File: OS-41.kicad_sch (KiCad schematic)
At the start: 65 parts, among them J1 Conn_02x03_Counter_Clockwise, J2 Conn_01x02_Pin, J3 Conn_01x02_Pin, J4 Conn_Coaxial, SW4 SW_Push, U1 BME280, U2 SI4432-B1-FMR, U3 MCP1640x-xCHY, U4 ATGM336H-5N31, U7 STM32F103C8Tx, Y1 32.768KHz 12.5pF, Y2 8MHz 12pF, Y3 30MHz 10pF

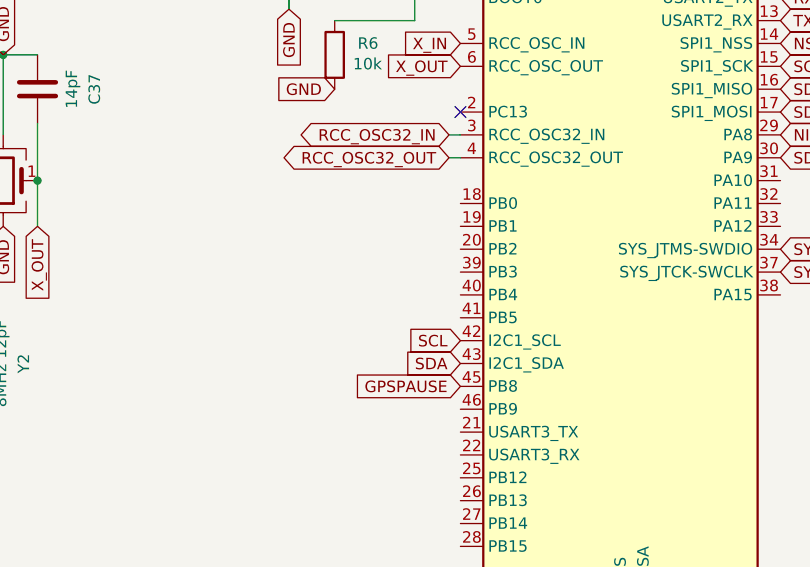
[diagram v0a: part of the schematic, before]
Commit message: Routed first version!
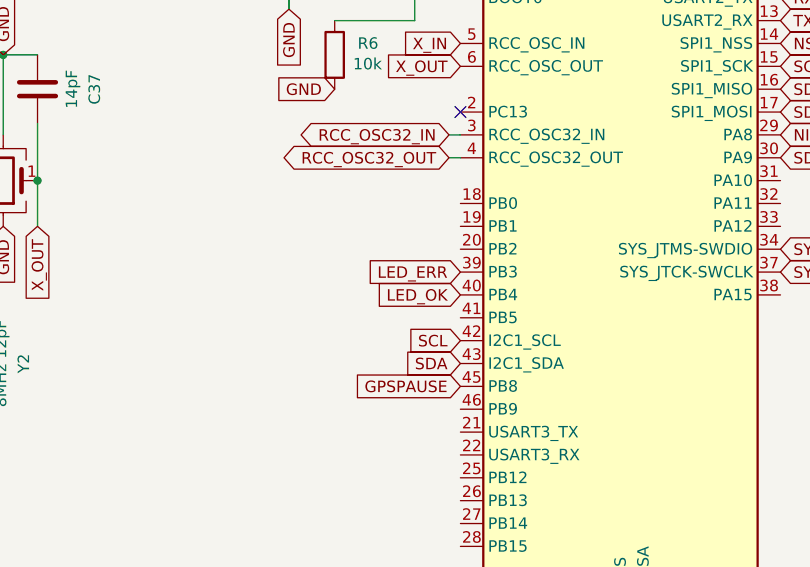
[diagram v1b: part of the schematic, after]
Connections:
- net LED_ERR: now also U7.39 (PB3)
- net LED_OK: now also U7.40 (PB4)
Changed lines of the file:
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@@
+		)
+	)
+	(global_label "LED_ERR"
+		(shape input)
+		(at 290.83 91.44 180)
+		(fields_autoplaced yes)
+		(effects
+			(font
+				(size 1.27 1.27)
+			)
+			(justify right)
+		)
+		(property "Intersheetrefs" "${INTERSHEET_REFS}"
+			(at 279.7411 91.44 0)
+			(effects
+				(font
+					(size 1.27 1.27)
+				)
+				(justify right)
+				(hide yes)
+			)
 		)
 	)
@@
 			(effects
 				(font
+					(size 1.27 1.27)
+				)
+				(justify right)
+				(hide yes)
+			)
+		)
+	)
+	(global_label "LED_OK"
+		(shape input)
+		(at 290.83 93.98 180)
+		(fields_autoplaced yes)
+		(effects
+			(font
+				(size 1.27 1.27)
+			)
+			(justify right)
+		)
+		(property "Intersheetrefs" "${INTERSHEET_REFS}"
+			(at 280.8296 93.98 0)
+			(effects
+				(font

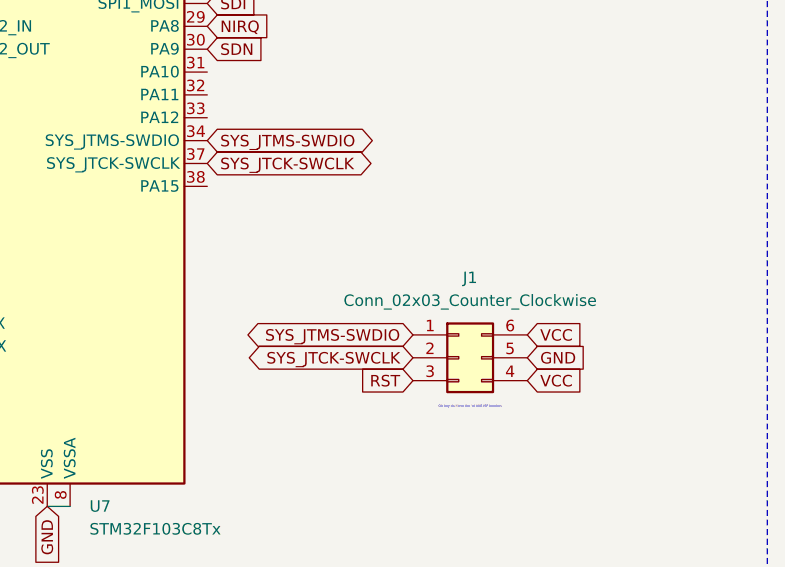
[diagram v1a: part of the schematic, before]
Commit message: More routing!
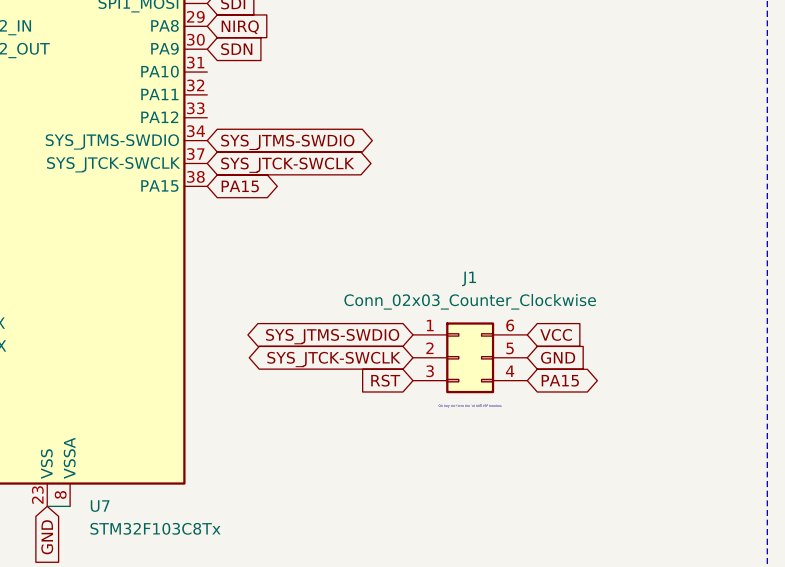
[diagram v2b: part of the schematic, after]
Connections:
- net VCC: no longer J1.4 (Pin_4)
- net PA15: now reaches U7.38 (PA15)
- net PA15: now also J1.4 (Pin_4)
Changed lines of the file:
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@@
+		)
+	)
+	(global_label "PA15"
+		(shape bidirectional)
+		(at 361.95 115.57 0)
+		(effects
+			(font
+				(size 1.27 1.27)
+			)
+			(justify left)
+		)
+		(property "Intersheetrefs" "${INTERSHEET_REFS}"
+			(at 361.95 115.57 0)
+			(effects
+				(font
+					(size 1.27 1.27)
+				)
+				(hide yes)
+			)
 		)
 	)
@@
 		)
 	)
-	(global_label "VCC"
-		(shape input)
-		(at 361.95 115.57 0)
-		(fields_autoplaced yes)
-		(effects
-			(font
-				(size 1.27 1.27)
-			)
-			(justify left)
-		)
-		(property "Intersheetrefs" "${INTERSHEET_REFS}"
-			(at 368.5638 115.57 0)
-			(effects
-				(font
-					(size 1.27 1.27)
-				)
-				(justify left)
-				(hide yes)
-			)
-		)
-	)
 	(global_label "SCL"
 		(shape input)
@@
 				(hide yes)
 			)
+		)
+	)
+	(global_label "PA15"
+		(shape bidirectional)
+		(at 326.39 93.98 0)
+		(effects
+			(font
+				(size 1.27 1.27)
+			)
+			(justify left)
+		)
+		(property "Intersheetrefs" "${INTERSHEET_REFS}"
+			(at 326.39 93.98 0)
+			(effects
+				(font
+					(size 1.27 1.27)
+				)
+				(hide yes)
+			)
